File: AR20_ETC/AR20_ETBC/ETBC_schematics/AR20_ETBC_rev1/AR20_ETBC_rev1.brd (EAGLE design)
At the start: 56 x 56 mm, 29 parts, among them J1 1-776267-1, X3 22-23-2021

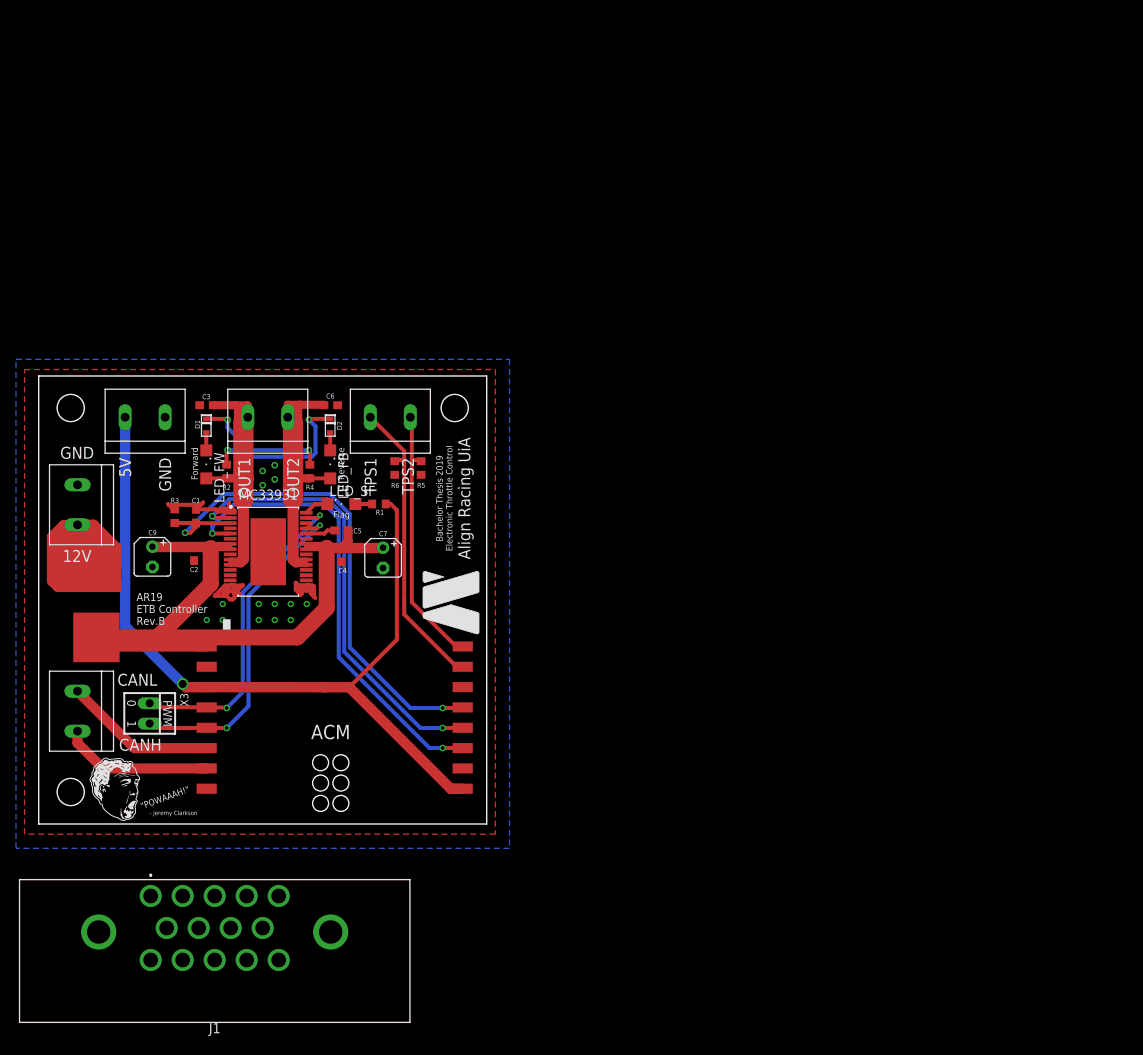
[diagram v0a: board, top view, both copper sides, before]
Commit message: .
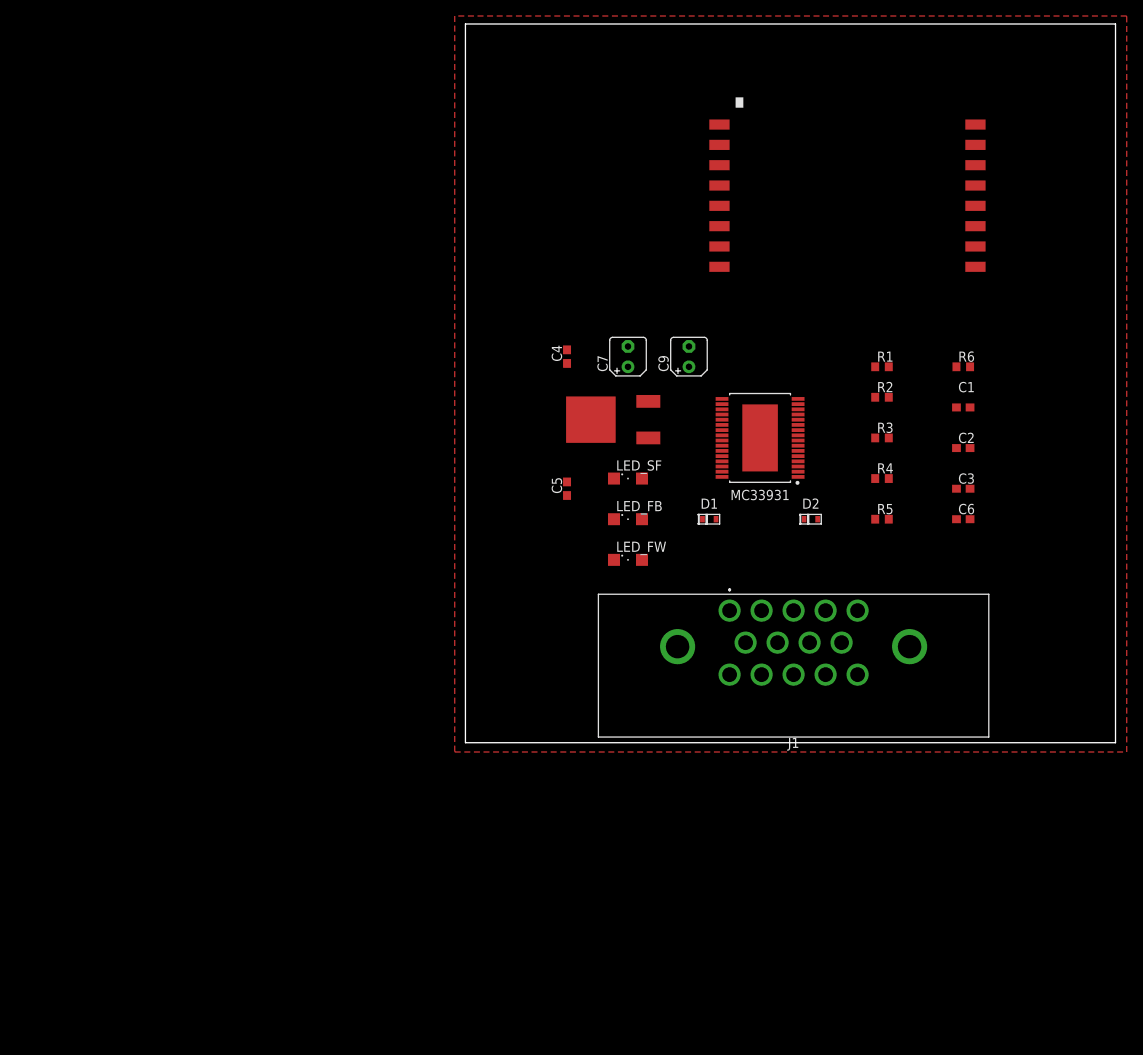
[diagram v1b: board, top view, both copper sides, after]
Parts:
- removed U$1, U$2, U$5, U$6, U$7: 2PIN_TERMINAL_BLOCK, AR19_ETC:2PIN_TERMINAL_BLOCK
- removed X3: 22-23-2021, con-molex:22-23-2021
- moved C2 97.1 mm to (115.6, 47.0), turned to 0 degrees
- moved C1 96.9 mm to (115.6, 52.1), turned to 0 degrees
- moved C3 95.2 mm to (115.6, 41.9), turned to 0 degrees
- moved U$3 91.5 mm to (85.1, 66.0)
- moved R3 88.9 mm to (105.4, 48.3), turned to 0 degrees
- moved R2 82.5 mm to (105.4, 53.3), turned to 0 degrees
- moved J1 80.7 mm to (86.4, 26.7)
- moved C6 80.3 mm to (115.6, 38.1)
- moved R6 72.2 mm to (115.6, 57.1), turned to 0 degrees
- moved C9 71.6 mm to (81.3, 58.4), turned to 90 degrees
- moved R4 71.5 mm to (105.4, 43.2), turned to 0 degrees
- moved D3 69.0 mm to (76.2, 48.3), turned to 0 degrees
- moved R1 65.2 mm to (105.4, 57.1)
- moved D1 64.0 mm to (83.8, 38.1), turned to 0 degrees
- moved MC33931 63.1 mm to (90.2, 48.3), turned to 180 degrees
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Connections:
- new net ECUTPS: J1.5
- new net N$16: J1.MH1
- new net N$22: J1.12
- new net N$24: J1.MH2
- new net SHUTD_IN: J1.8
- new net SHUTD_OUT: J1.9
- net 12V: now also J1.13; no longer U$2.P$1
- net 5V: now also J1.3; no longer U$6.P$1
- net CANH: now also J1.6; no longer U$1.P$1
- net CANL: now also J1.7; no longer U$1.P$2
- net GND: now also J1.14, J1.4; no longer U$2.P$2, U$6.P$2
- net OUT1: now also J1.10; no longer U$5.P$1
- net OUT2: now also J1.11; no longer U$5.P$2
- net PWM0: no longer X3.1
- net PWM1: no longer X3.2
- net TPS1: now also J1.1; no longer U$7.P$2
- net TPS2: now also J1.2; no longer U$7.P$1
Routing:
- net VPWR: track 107.7 -> 0.00 mm
- net 5V: track 103.1 -> 0.00 mm, vias 1 -> 0
- net 12V: track 96.9 -> 0.00 mm
- net FEEDBACK: track 67.0 -> 0.00 mm, vias 2 -> 0
- net ENABLE/D2: track 58.7 -> 0.00 mm, vias 2 -> 0
- net D1: track 56.6 -> 0.00 mm, vias 2 -> 0
- net GND: track 42.2 -> 0.00 mm, vias 4 -> 0
- net PWM1: track 42.2 -> 0.00 mm, vias 2 -> 0
- net PWM0: track 40.7 -> 0.00 mm, vias 2 -> 0
- net OUT2: track 39.8 -> 0.00 mm
- net OUT1: track 39.0 -> 0.00 mm
- net TPS2: track 37.7 -> 0.00 mm
- net TPS1: track 33.1 -> 0.00 mm
- net N$7: track 20.6 -> 0.00 mm, vias 2 -> 0
- net CANL: track 19.1 -> 0.00 mm
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- removed copper zone on layer 16, net GND
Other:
- board size 56 x 56 mm -> 81.3 x 89.8 mm
- board text removed: ""POWAAAH!""
- board text removed: "- Jeremy Clarkson"
- board text removed: "0"
- board text removed: "1"
- board text removed: "12V"
- board text removed: "5V"
- board text removed: "ACM"
- board text removed: "AR19 ETB Controller Rev.B"
- board text removed: "Align Racing UiA"
- board text removed: "Bachelor Thesis 2019 Electronic Throttle Control"
- board text removed: "CANH"
- board text removed: "CANL"
- board text removed: "Flag"
- board text removed: "Forward"
- board text removed: "GND"
- board text removed: "OUT1"
- board text removed: "OUT2"
- board text removed: "PWM"
- board text removed: "Reverse"
- board text removed: "TPS1"
- board text removed: "TPS2"
